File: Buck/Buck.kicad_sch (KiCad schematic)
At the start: 32 parts, among them IC1 LM5148RGYR

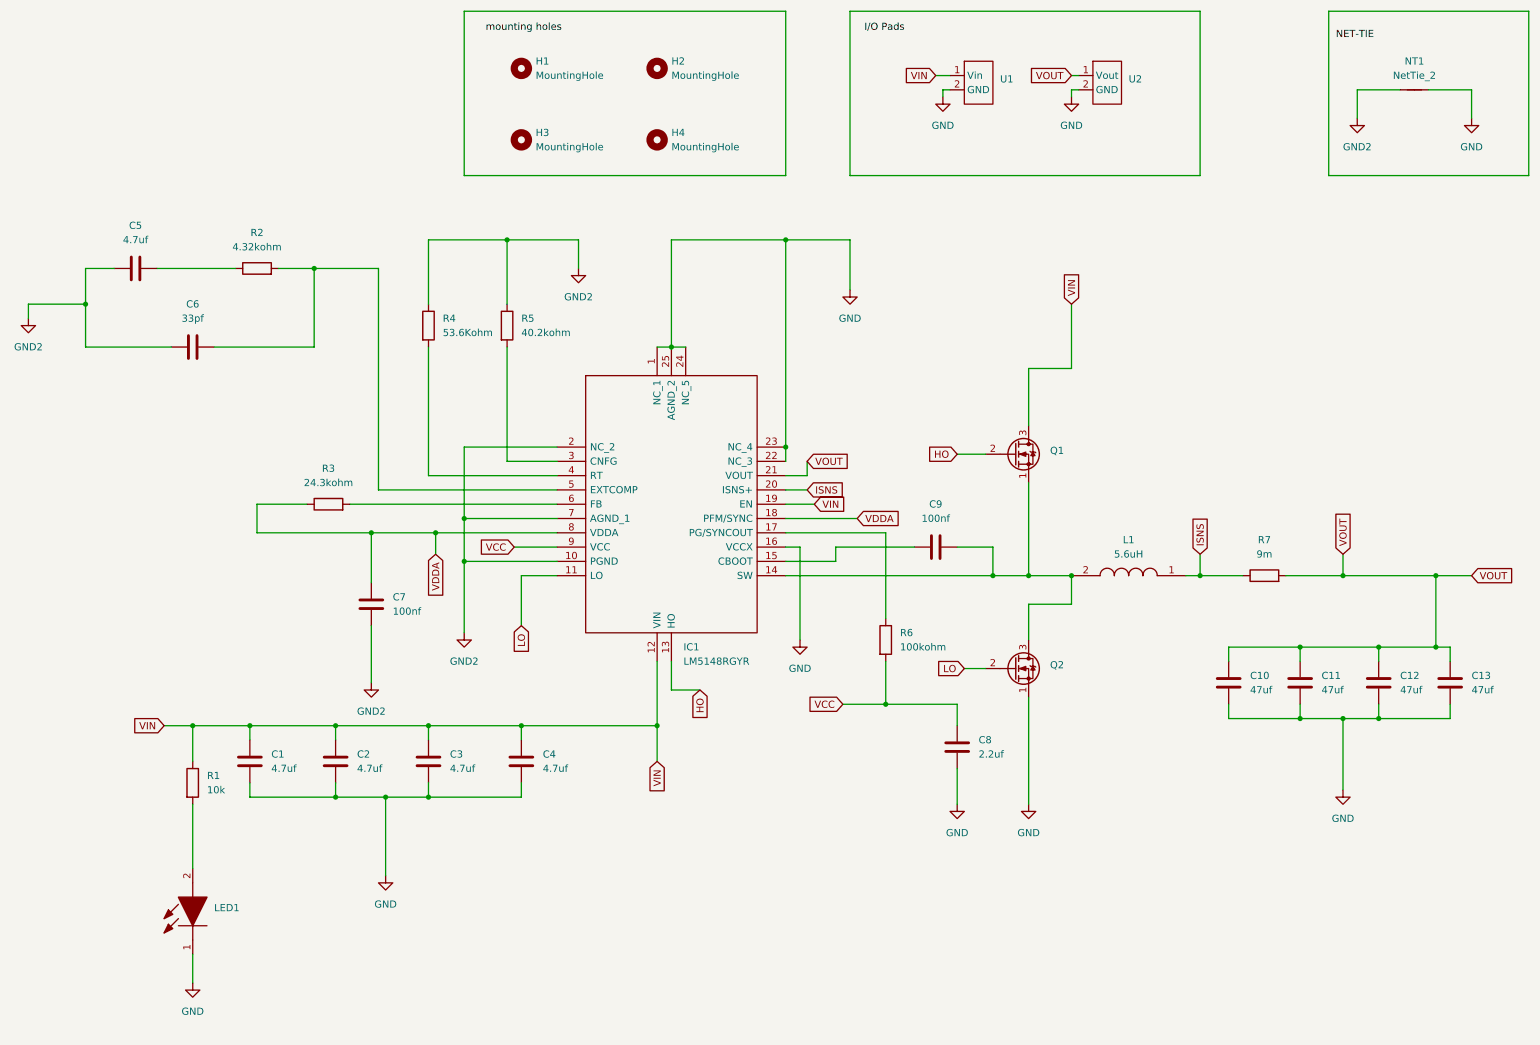
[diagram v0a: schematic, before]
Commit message: Updated
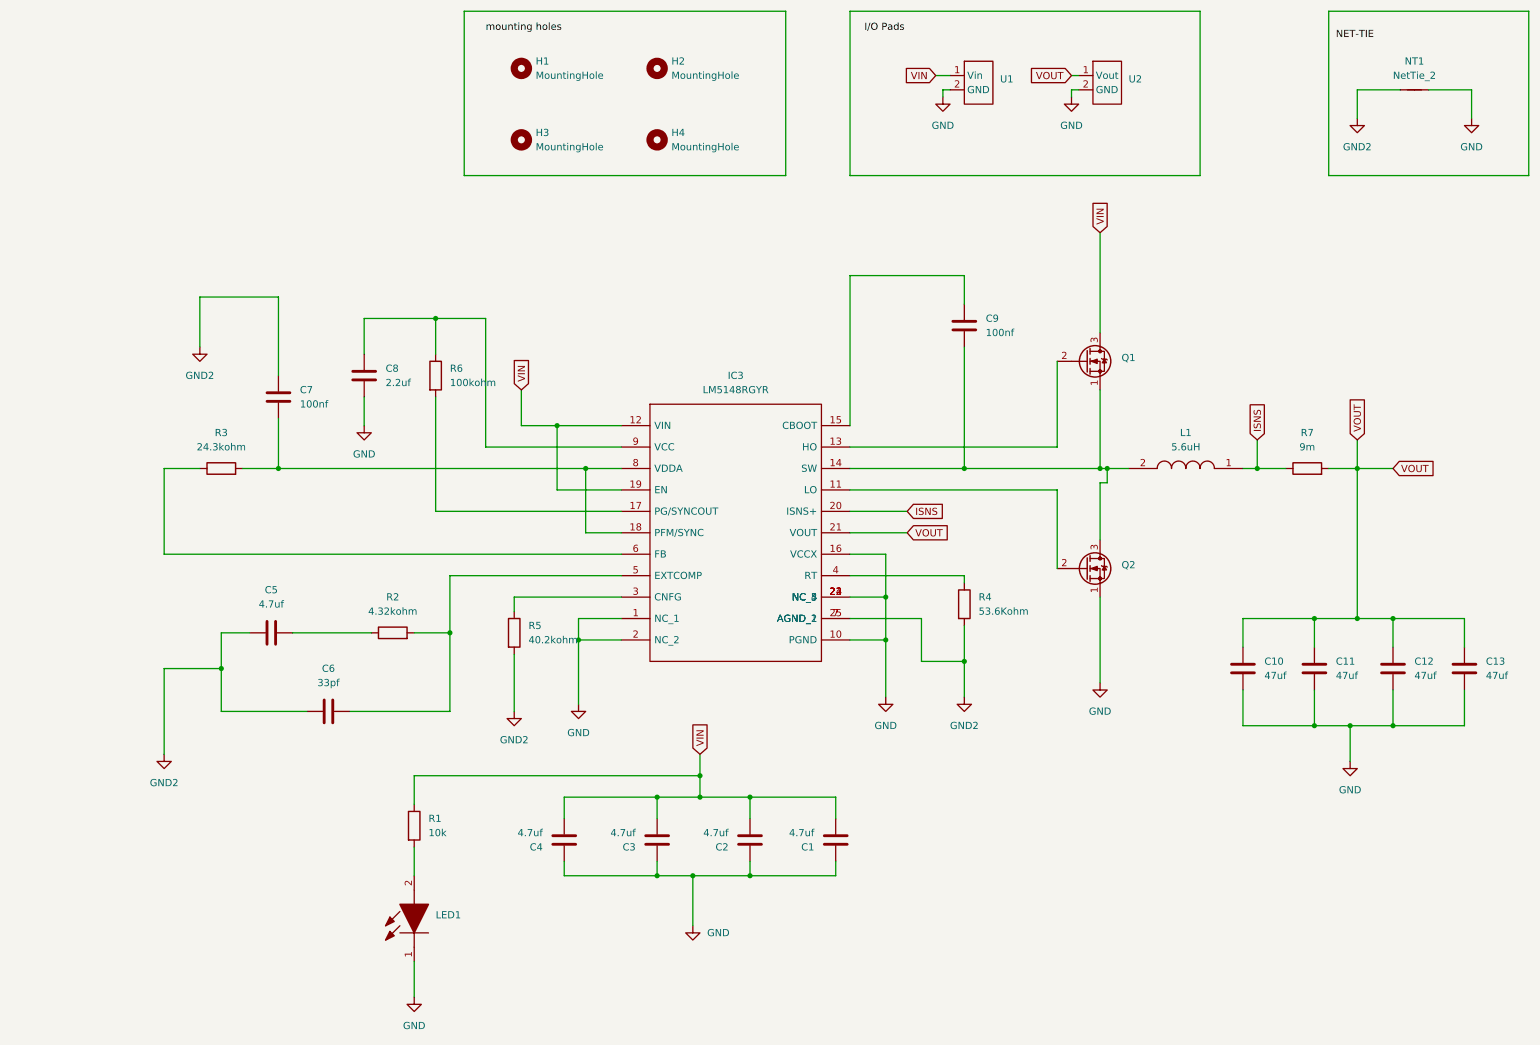
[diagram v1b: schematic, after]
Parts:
- removed IC1: LM5148RGYR, LM5148_:LM5148RGYR, symbol LM5148RGYR:LM5148RGYR
- added IC3: LM5148RGYR, LM5148RGYR, symbol LM5148RGYR_edited normal_symbol:LM5148RGYR
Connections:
- net GND: now also C1.1, C2.1, C3.1, C4.1, IC3.1 (NC_1), IC3.10 (PGND), IC3.16 (VCCX), IC3.2 (NC_2), IC3.22 (NC_3), IC3.23 (NC_4), IC3.24 (NC_5); no longer C1.2, C2.2, C3.2, C4.2
- net GND2: now also C7.1, R4.2, R5.2, IC3.25 (AGND_2), IC3.7 (AGND_1); no longer C7.2, R4.1, R5.1
- net ISNS: now also IC3.20 (ISNS+)
- net VIN: now also C1.2, C2.2, C3.2, C4.2, IC3.12 (VIN), IC3.19 (EN); no longer C1.1, C2.1, C3.1, C4.1
- net VOUT: now also IC3.21 (VOUT)
- net at L1.2, Q1.1 (S), Q2.3 (D): now also C9.1, IC3.14 (SW); no longer C9.2
- net at R6.1: now also C8.1, IC3.9 (VCC)
- net at C6.1, R2.2: now also IC3.5 (EXTCOMP)
- net at R3.2: now also C7.2, IC3.18 (PFM/SYNC), IC3.8 (VDDA)
- net HO: no longer names the net of Q1.2 (G)
- net HO: now also IC3.13 (HO)
- net LO: no longer names the net of Q2.2 (G)
- net LO: now also IC3.11 (LO)
- net VCC: no longer names the net of R6.2
- net VCC: now also IC3.17 (PG/SYNCOUT); no longer C8.1
- net VDDA: no longer names the net of R3.1
- net VDDA: now also IC3.6 (FB); no longer C7.1
- new net: C9.2, IC3.15 (CBOOT)
- new net: IC3.3 (CNFG), R5.1
- new net: IC3.4 (RT), R4.1
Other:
- moved on the sheet: C1, C10, C11, C12, C13, C2, C3, C4, C5, C6, C7, C8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
